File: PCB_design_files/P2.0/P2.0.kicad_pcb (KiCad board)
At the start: 4 copper layers, 19 x 19 mm, 59 parts, among them J1 EEG_IN, J2 20021121-00008C4LF, U1 INA819IDRGR, U2 TLV9102IDSGR, U3 TPS61094, U4 TPS60400, U5 NRF52832-QFAA-R, Y1 32MHz

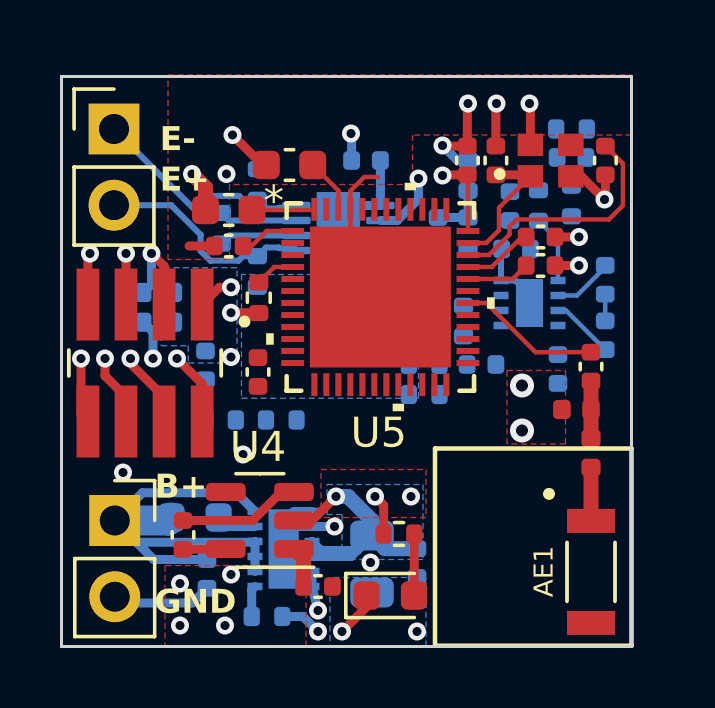
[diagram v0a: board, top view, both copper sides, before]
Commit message: Updated schematic
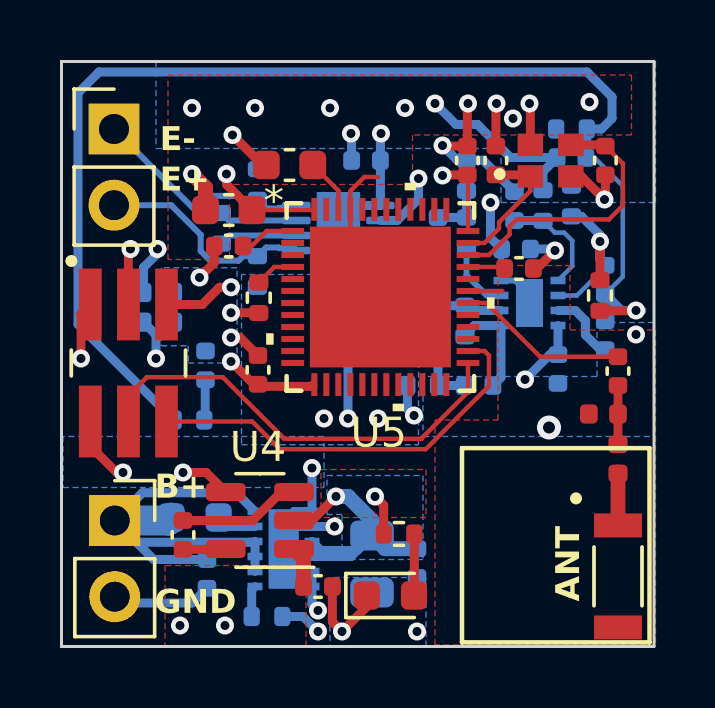
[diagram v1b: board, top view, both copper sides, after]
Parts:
- removed C21: ~, Capacitor_SMD:C_0402_1005Metric
- J2: value 20021121-00008C4LF -> Conn_02x03_Counter_Clockwise; footprint 20021121_00008C4LF:AMPHENOL_20021121-00008C4LF -> 20021121_00006C4LF:AMPHENOL_20021121-00006C4LF
- R13: moved to F.Cu
- moved R13 11.4 mm to (92.7, 57.3), turned to -90 degrees
- moved C17 1.27 mm to (90.0, 56.4)
- moved R14 1.05 mm to (79.0, 61.5), turned to 0 degrees
- moved L2 0.92 mm to (93.3, 62.7)
- moved C15 0.91 mm to (93.3, 59.8)
- moved L3 0.91 mm to (92.8, 61.2)
- moved AE1 0.91 mm to (93.3, 66.7)
- moved C2 0.71 mm to (88.7, 60.3)
- moved J2 0.56 mm to (77.0, 59.5), turned to 0 degrees
- moved R10 0.30 mm to (86.8, 60.3)
- moved R9 0.30 mm to (86.8, 59.3)
- moved C4 0.15 mm to (89.8, 54.3)
- moved R11 0.15 mm to (90.8, 54.3)
- moved C14 0.07 mm to (81.3, 59.8)
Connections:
- J2 pad 1: STAGE_3_OUT -> -3V3
- J2 pad 3: GND -> STAGE_3_OUT
- J2 pad 4: -3V3 -> SWDIO
- J2 pad 5: NRST -> SWDCLK
- J2 pad 6: SWO -> GND
- U3 pad 13: (no net) -> GND
- U5 pad 21: SWO -> unconnected-(U5-P0.18/TRACEDATA[0]/SWO-Pad21)
- U5 pad 24: NRST -> unconnected-(U5-P0.21/Nreset-Pad24)
- U5 pad 32: Net-(U5-DEC2) -> unconnected-(U5-DEC2-Pad32)
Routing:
- net -3V3: track 8.80 -> 50.8 mm, vias 4 -> 5
- net Net-(C3-Pad2): track 0.89 -> 42.3 mm, vias 0 -> 1
- net Net-(C5-Pad1): track 0.00 -> 25.8 mm, vias 0 -> 2
- net SWDCLK: track 2.56 -> 14.9 mm, vias 1 -> 0
- net +3V3: track 21.6 -> 33.7 mm, vias 6 -> 9
- net GND: track 37.0 -> 48.8 mm, vias 25 -> 31
- net SWDIO: track 2.45 -> 13.8 mm, vias 1 -> 0
- net Net-(U2-IN2-): track 2.03 -> 5.61 mm, vias 0 -> 1
- net Net-(U2-OUT1): track 0.00 -> 3.51 mm
- net SWO: track 2.39 -> 0.00 mm, vias 1 -> 0
- net Net-(U2-IN1+): track 0.00 -> 2.33 mm
- net Net-(U2-IN1-): track 0.00 -> 2.21 mm
- net NRST: track 2.20 -> 0.00 mm, vias 1 -> 0
- net Net-(U5-DEC2): track 2.13 -> 0.00 mm
- net Net-(C2-Pad2): track 0.00 -> 1.87 mm
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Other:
- board size 19 x 19 mm -> 19.8 x 19.5 mm
- board text added: "ANT"
- board text added: "JY-68 P2.0"
